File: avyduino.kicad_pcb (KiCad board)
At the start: 2 copper layers, 68.6 x 53.3 mm, 38 parts, among them J1 Power, J2 Digital/PWM, J3 Analog, J4 Digital/PWM, J5 USB_C_Receptacle_USB2.0_14P, Q1 AO3401A, U1 ATmega328P-P, U2 CH340G, U3 LM2931AZ-5.0_TO92, U4 MCP1700x-330xxTT, U5 LM358, Y1 12MHz, Y2 16MHz

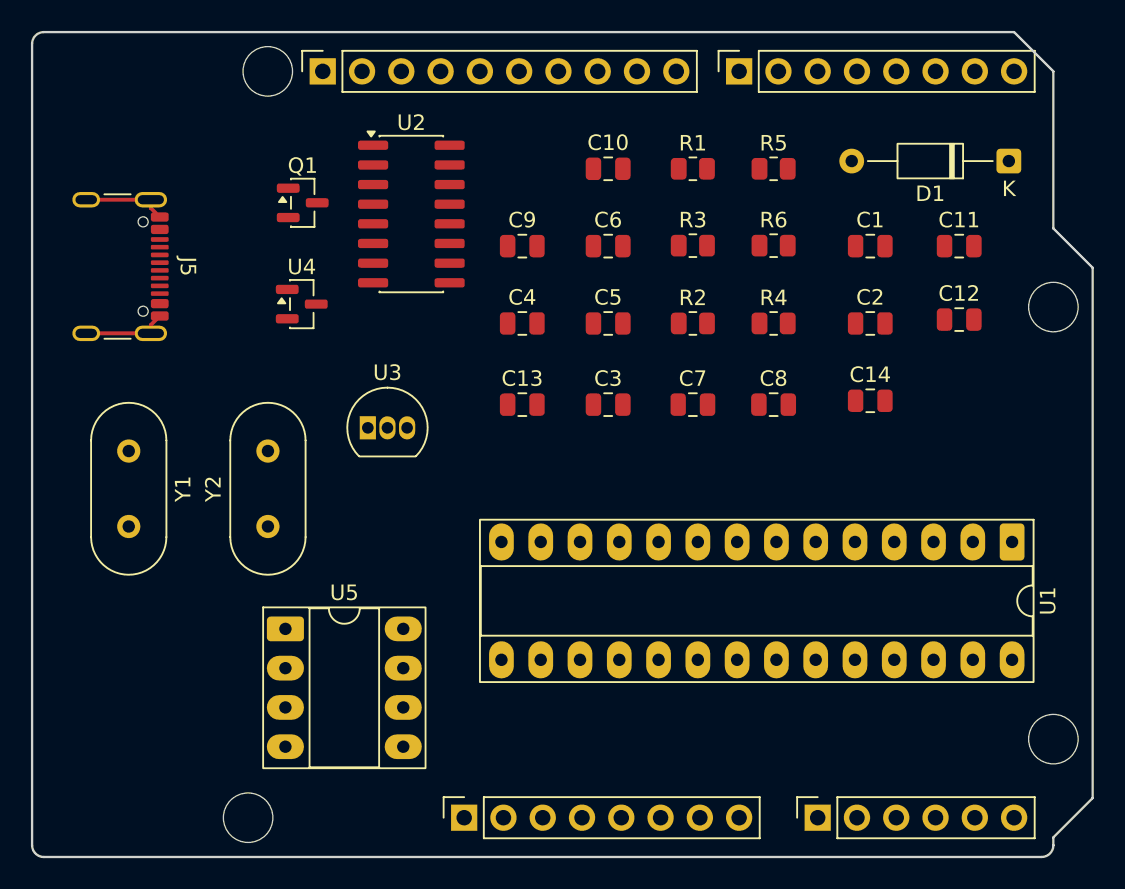
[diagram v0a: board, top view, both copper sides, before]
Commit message: route the pcb. will add some cool silkscreen
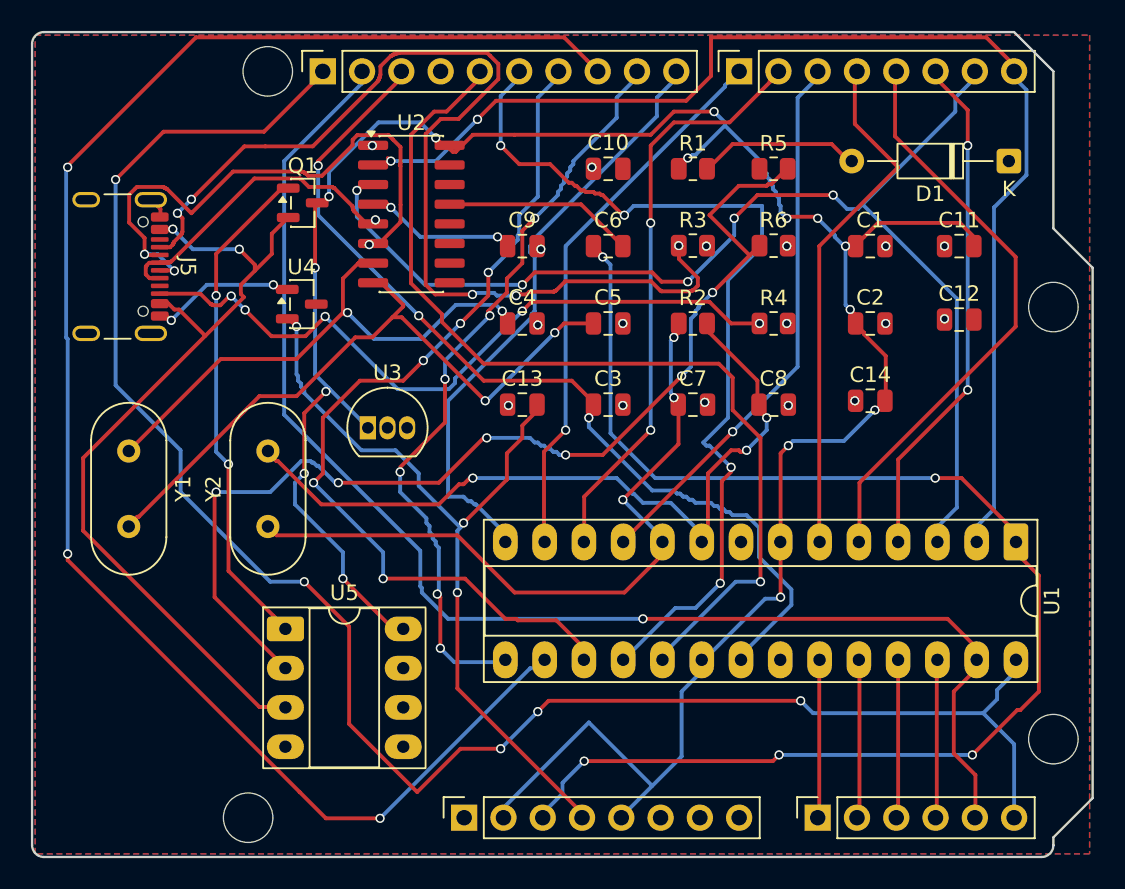
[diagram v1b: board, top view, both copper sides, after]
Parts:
- moved U1 0.25 mm to (163.6, 79.6)
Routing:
- net +5V: track 0.00 -> 154.3 mm, vias 0 -> 15
- net /SCL/A5: track 0.00 -> 116.2 mm, vias 0 -> 5
- net /*10: track 0.00 -> 105.9 mm, vias 0 -> 3
- net /SDA/A4: track 0.00 -> 88.5 mm, vias 0 -> 1
- net /~{RESET}: track 0.00 -> 88.0 mm, vias 0 -> 5
- net /RX/0: track 0.00 -> 77.8 mm, vias 0 -> 2
- net /TX/1: track 0.00 -> 77.4 mm, vias 0 -> 5
- net Net-(U5A--): track 0.00 -> 68.7 mm, vias 0 -> 6
- net Net-(J5-CC1): track 0.00 -> 67.6 mm, vias 0 -> 5
- net /13: track 0.00 -> 61.6 mm, vias 0 -> 1
- net /AREF: track 0.00 -> 60.3 mm, vias 0 -> 3
- net /12: track 0.00 -> 58.7 mm, vias 0 -> 4
- net /*11: track 0.00 -> 58.0 mm, vias 0 -> 5
- net VBUS: track 0.00 -> 55.2 mm, vias 0 -> 2
- net +3V3: track 0.00 -> 51.4 mm, vias 0 -> 3
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- added copper zone on B.Cu, net GND
- added copper zone on F.Cu, net VCC
